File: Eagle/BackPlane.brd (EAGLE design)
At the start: 99.7 x 99.1 mm, 34 parts, among them IC2 REG1117, IC4 DS1813, IC5 DS1813, J1 DCJ0202

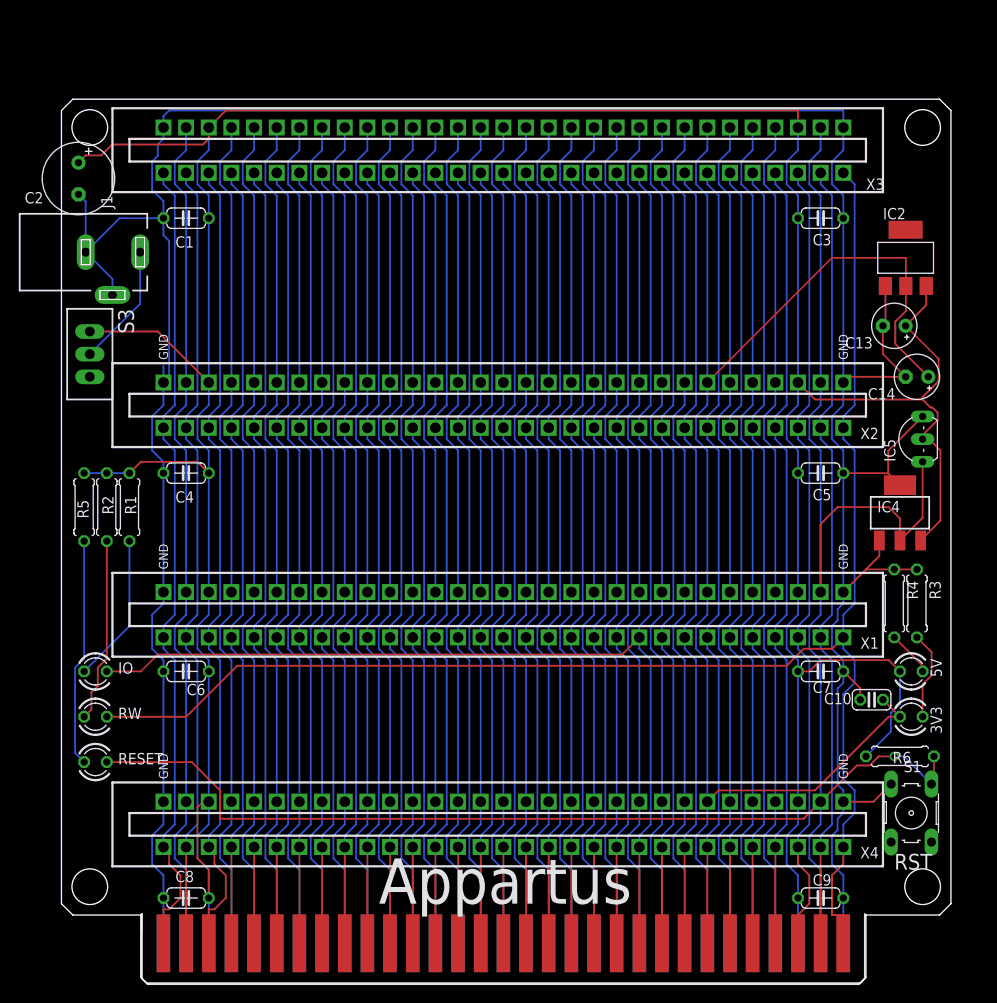
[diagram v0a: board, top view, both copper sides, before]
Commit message: Init
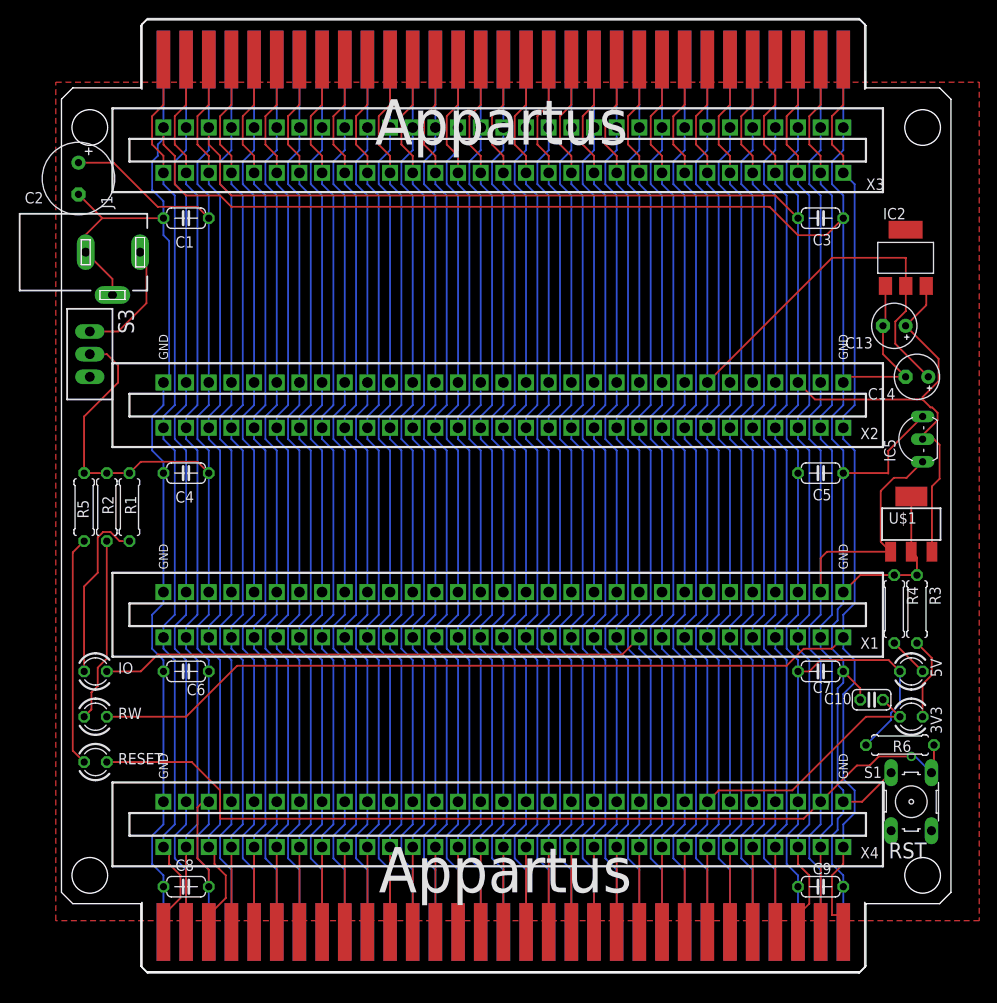
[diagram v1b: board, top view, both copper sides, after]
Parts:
- removed IC4: DS1813, ds1813_revised:SOT223
- added U$1: DS1233SOT223, TiRoRiN_Libs:SOT223
- ST1: device TiRoRiN_Libs:APP_2X32_SHORT -> TiRoRiN_Libs:APP_2X32_DOUBLE
- moved C8 1.27 mm to (20.3, 13.3)
- moved C9 1.27 mm to (91.4, 13.3)
- moved R6 1.27 mm to (100.3, 29.2)
- moved S1 1.27 mm to (101.6, 22.9)
- moved R3 0.63 mm to (102.2, 44.5)
- moved R4 0.63 mm to (99.7, 44.5)
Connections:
- net +3V3: now also ST1.B38
- net +5V: now also S3.2, ST1.B34, ST1.B60, U$1.3; no longer IC4.3, S3.1
- net CLK: now also ST1.B61
- net GND: now also ST1.B32, ST1.B62, U$1.2, U$1.4; no longer IC4.1, IC4.4
- net IO_SEL: now also ST1.A41
- net N$12: now also ST1.A42
- net N$13: now also ST1.A43
- net N$14: now also ST1.A44
- net N$15: now also ST1.A45
- net N$16: now also ST1.A46
- net N$17: now also ST1.A47
- net N$18: now also ST1.A48
- net N$19: now also ST1.A49
- net N$2: now also ST1.A33
- net N$20: now also ST1.A50
- net N$21: now also ST1.A51
- net N$22: now also ST1.A52
- net N$23: now also ST1.A53
- net N$24: now also ST1.A54
- net N$25: now also ST1.A55
- net N$26: now also ST1.A56
- net N$27: now also ST1.A57
- net N$28: now also ST1.A58
- net N$29: now also ST1.A59
- net N$3: now also ST1.A34
- net N$30: now also ST1.A60
- net N$31: now also ST1.A61
- net N$32: now also ST1.A62
- net N$35: now also ST1.B35
- net N$36: now also ST1.B36
- net N$37: now also ST1.B37
- net N$39: now also ST1.B39
- net N$4: now also ST1.A35
- net N$40: now also ST1.B40
- net N$41: now also ST1.B41
- net N$42: now also ST1.B42
- net N$43: now also ST1.B43
- net N$44: now also ST1.B44
- net N$45: now also ST1.B45
- net N$46: now also ST1.B46
- net N$47: now also ST1.B47
- net N$48: now also ST1.B48
- net N$49: now also ST1.B49
- net N$5: now also ST1.A36
- net N$50: now also ST1.B50
- net N$51: now also ST1.B51
- net N$52: now also ST1.B52
- net N$53: now also ST1.B53
- net N$54: now also ST1.B54
- net N$55: now also ST1.B55
- net N$56: now also ST1.B56
- net N$57: now also ST1.B57
- net N$58: now also ST1.B58
- net N$59: now also ST1.B59
- net N$6: now also ST1.A37
- net N$7: now also ST1.A38
- net N$8: now also ST1.A39
- net N$9: now also ST1.A40
- net RESET: now also ST1.B33, U$1.1; no longer IC4.2
- net RW: now also ST1.A32
- net VCC: now also S3.1; no longer S3.2
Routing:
- net GND: track 354.5 -> 372.3 mm
- net +5V: track 394.1 -> 411.2 mm
- net N$3: track 90.6 -> 103.1 mm
- net N$13: track 89.5 -> 102.0 mm
- net RW: track 178.6 -> 191.1 mm
- net N$9: track 89.5 -> 102.0 mm
- net N$8: track 89.5 -> 102.0 mm
- net N$7: track 89.5 -> 102.0 mm
- net N$6: track 89.5 -> 102.0 mm
- net N$5: track 89.5 -> 102.0 mm
- net N$4: track 89.5 -> 102.0 mm
- net N$31: track 89.5 -> 102.0 mm
- net N$29: track 89.5 -> 102.0 mm
- net N$28: track 89.5 -> 102.0 mm
- net N$27: track 89.5 -> 102.0 mm
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- added copper zone on layer 1, net GND
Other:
- board size 99.7 x 99.1 mm -> 99.7 x 106.7 mm
